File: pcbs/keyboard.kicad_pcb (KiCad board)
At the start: 2 copper layers, 178 x 136.4 mm, 106 parts, among them J1 Jumper, J10 Jumper, J11 Jumper, J12 Jumper, J13 Jumper, J14 Jumper, J15 Jumper, J16 Jumper, J17 Jumper, J18 Jumper, J2 Jumper, J3 Jumper, J4 Jumper, J5 Jumper, J6 Jumper, J7 Jumper, J8 Jumper, J9 Jumper

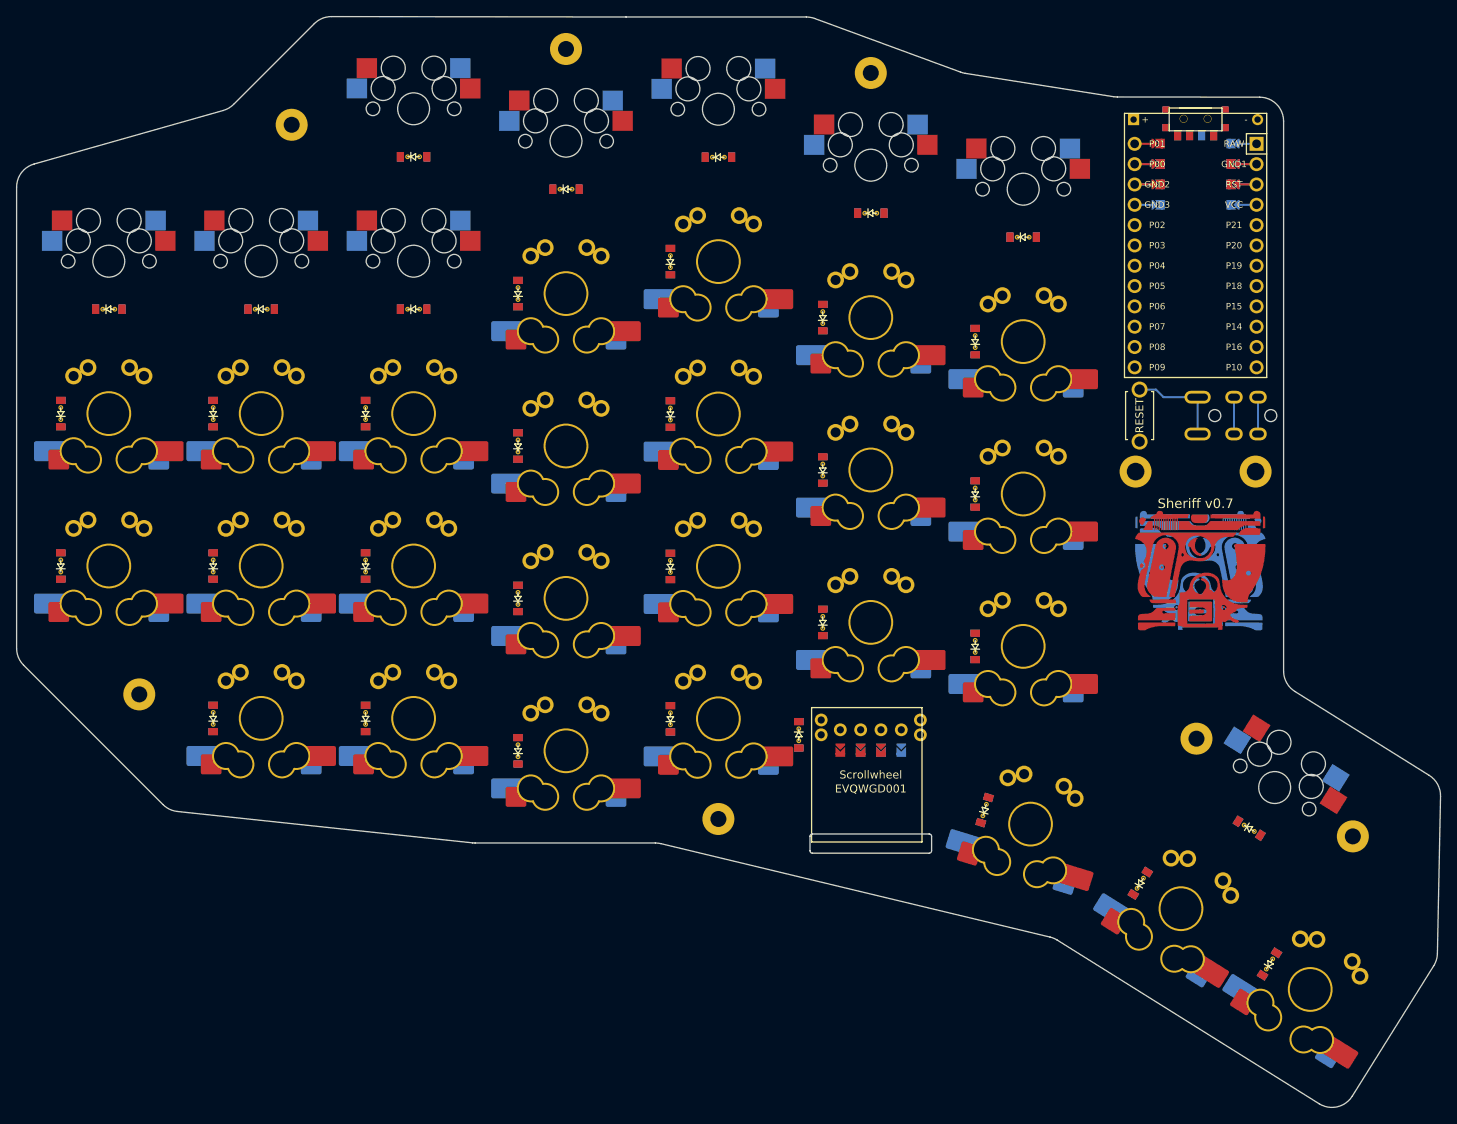
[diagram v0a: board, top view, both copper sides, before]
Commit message: routed pcb
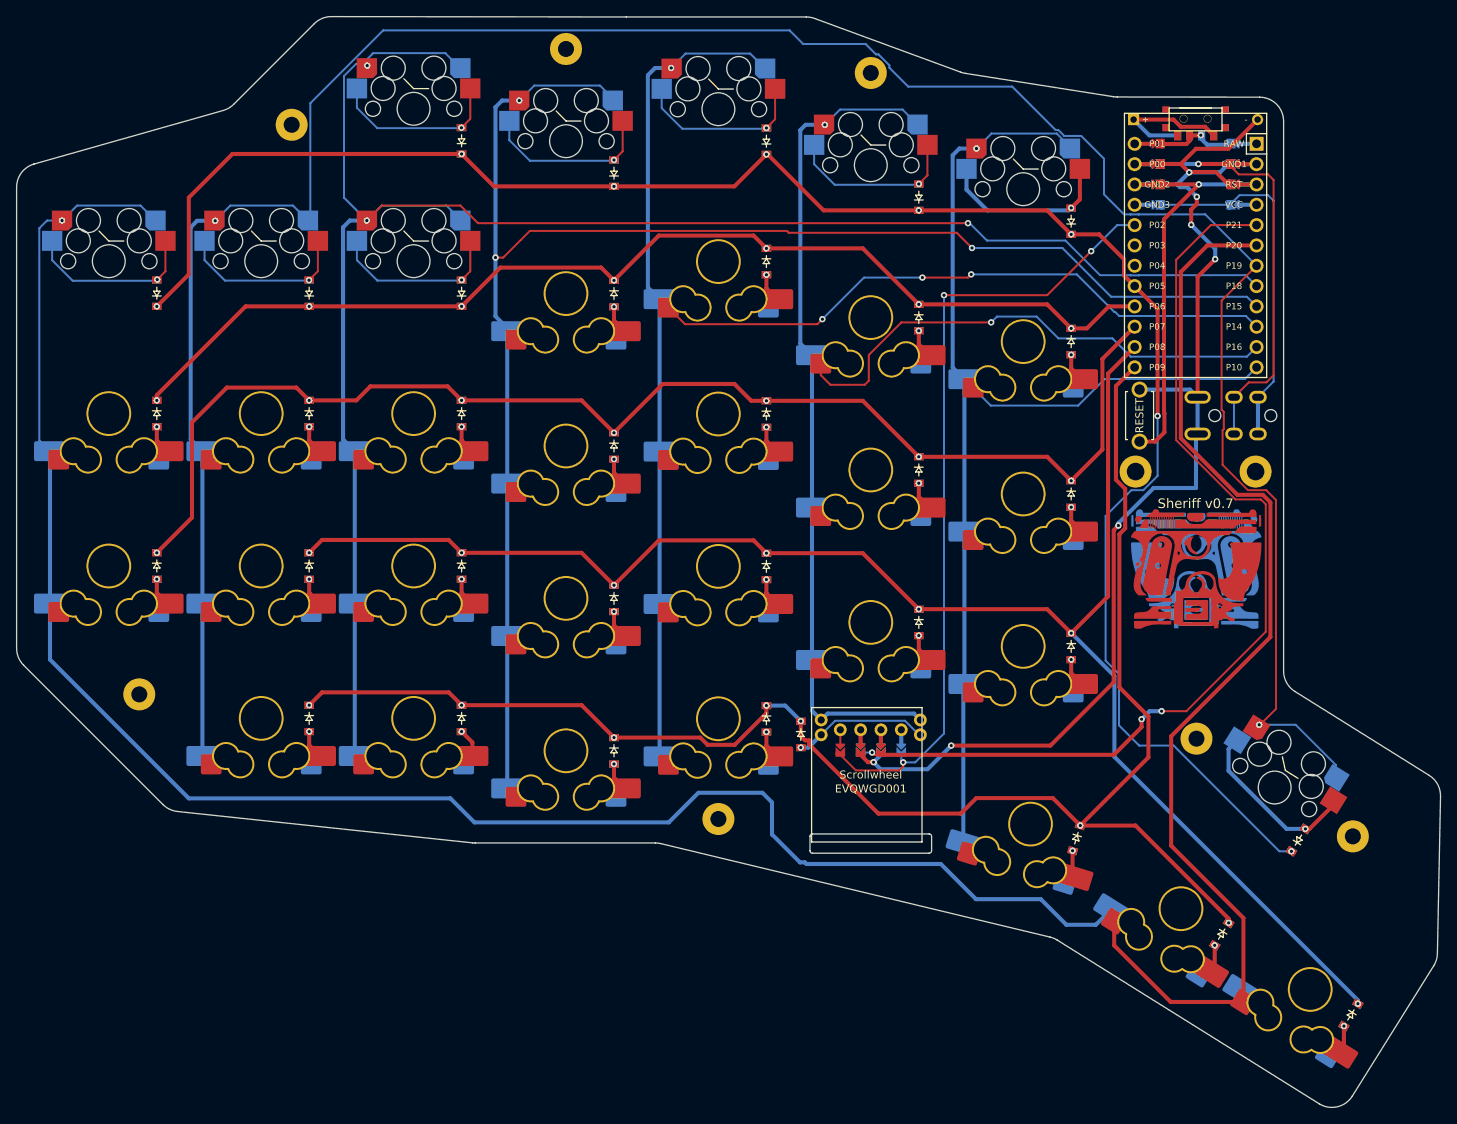
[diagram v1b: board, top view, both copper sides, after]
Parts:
- removed the ? at (185.8, 123.2) (x2)
- removed the G*** at (187.0, 131.0)
- removed the G*** at (185.9, 131.0)
- added ? (x2): , lib:text, F.Cu at (185.8, 123.2)
- added G***: LOGO, Custom:Logo, F.Cu at (186.5, 130.8)
- added G***: LOGO, Custom:Logo, B.Cu at (185.4, 130.8)
- D1, D10, D11, D12, D13, D14, D15, D16, D17, D18, D19, D2, D20, D21, D22, D23, D24, D25, D26, D27, D28, D29, D3, D30, D31, D32, D33, D34, D4, D5, D6, D7, D8, D9: footprint ComboDiode -> ceoloide:diode_tht_sod123; moved to B.Cu
- S26, S27, S28, S29, S30, S31, S32, S33, S34: footprint MX -> ceoloide:switch_mx; moved to B.Cu
- moved D25 12.0 mm to (205.3, 187.1), turned to -122 degrees
- moved D24 12.0 mm to (189.1, 177.0), turned to -122 degrees
- moved D1 12.0 mm to (56.0, 130.9), turned to -90 degrees
- moved D10 12.0 mm to (113.2, 135.0), turned to -90 degrees
- moved D11 12.0 mm to (113.2, 116.0), turned to -90 degrees
- moved D12 12.0 mm to (113.2, 96.9), turned to -90 degrees
- moved D17 12.0 mm to (151.2, 138.0), turned to -90 degrees
- moved D18 12.0 mm to (151.2, 119.0), turned to -90 degrees
- moved D19 12.0 mm to (151.2, 99.9), turned to -90 degrees
- moved D2 12.0 mm to (56.0, 111.9), turned to -90 degrees
- moved D20 12.0 mm to (170.3, 141.0), turned to -90 degrees
- moved D21 12.0 mm to (170.3, 122.0), turned to -90 degrees
- moved D22 12.0 mm to (170.3, 102.9), turned to -90 degrees
- moved D3 12.0 mm to (75.0, 150.0), turned to -90 degrees
- moved D4 12.0 mm to (75.0, 130.9), turned to -90 degrees
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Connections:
- D12 pad 1: row2 -> row1
- D16 pad 1: row2 -> row1
- D19 pad 1: row2 -> row1
- D22 pad 1: row2 -> row1
- D27 pad 1: row2 -> row1
- D28 pad 1: row2 -> row1
- S26 pad 1: col0 -> outer2_top
- S26 pad 2: outer2_top -> col0
- S27 pad 1: col1 -> outer1_top
- S27 pad 2: outer1_top -> col1
- S28 pad 1: col2 -> pinky_top
- S28 pad 2: pinky_top -> col2
- S29 pad 1: col2 -> pinky_num
- S29 pad 2: pinky_num -> col2
- S30 pad 1: col3 -> ring_num
- S30 pad 2: ring_num -> col3
- S31 pad 1: col4 -> middle_num
- S31 pad 2: middle_num -> col4
- S32 pad 1: col5 -> index_num
- S32 pad 2: index_num -> col5
- S33 pad 1: col6 -> inner_num
- S33 pad 2: inner_num -> col6
- S34 pad 1: col1 -> home_high
- S34 pad 2: home_high -> col1
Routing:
- net col0: track 0.00 -> 363.1 mm, vias 0 -> 1
- net col1: track 0.00 -> 313.3 mm, vias 0 -> 2
- net col2: track 0.00 -> 238.2 mm, vias 0 -> 3
- net row0: track 0.00 -> 235.5 mm, vias 0 -> 8
- net row3: track 0.00 -> 205.6 mm, vias 0 -> 7
- net col3: track 0.00 -> 203.1 mm, vias 0 -> 3
- net row4: track 0.00 -> 199.5 mm, vias 0 -> 7
- net col4: track 0.00 -> 182.0 mm, vias 0 -> 4
- net col5: track 0.00 -> 168.8 mm, vias 0 -> 2
- net row2: track 0.00 -> 163.7 mm, vias 0 -> 7
- net col6: track 0.00 -> 143.2 mm, vias 0 -> 1
- net row1: track 0.00 -> 138.4 mm, vias 0 -> 7
- net GND: track 12.2 -> 149.9 mm, vias 0 -> 7
- net ENCA: track 0.00 -> 122.7 mm, vias 0 -> 3
- net ENCB: track 0.00 -> 99.3 mm, vias 0 -> 3
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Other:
- outline, holes or cut-outs redrawn
